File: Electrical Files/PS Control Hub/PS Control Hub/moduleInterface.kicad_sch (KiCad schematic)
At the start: 4 parts, among them K1 Relay_SPST-NO

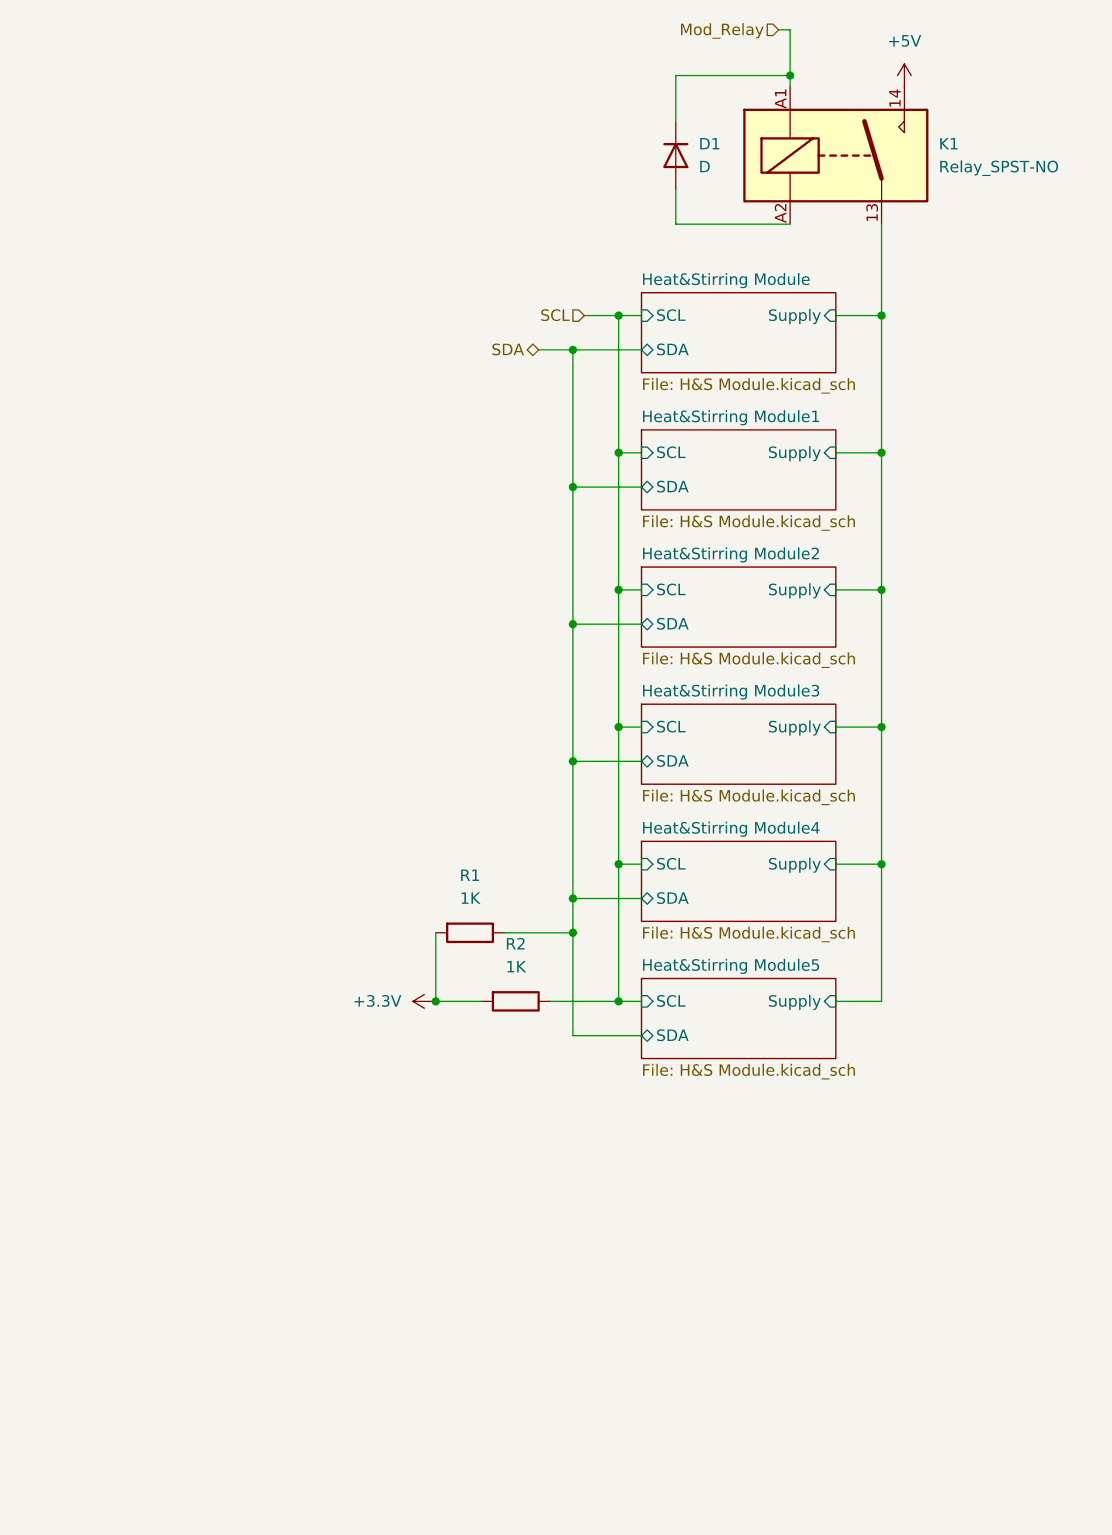
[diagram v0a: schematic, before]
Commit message: Control Hub, Flexible Hotplate, Housing Fan
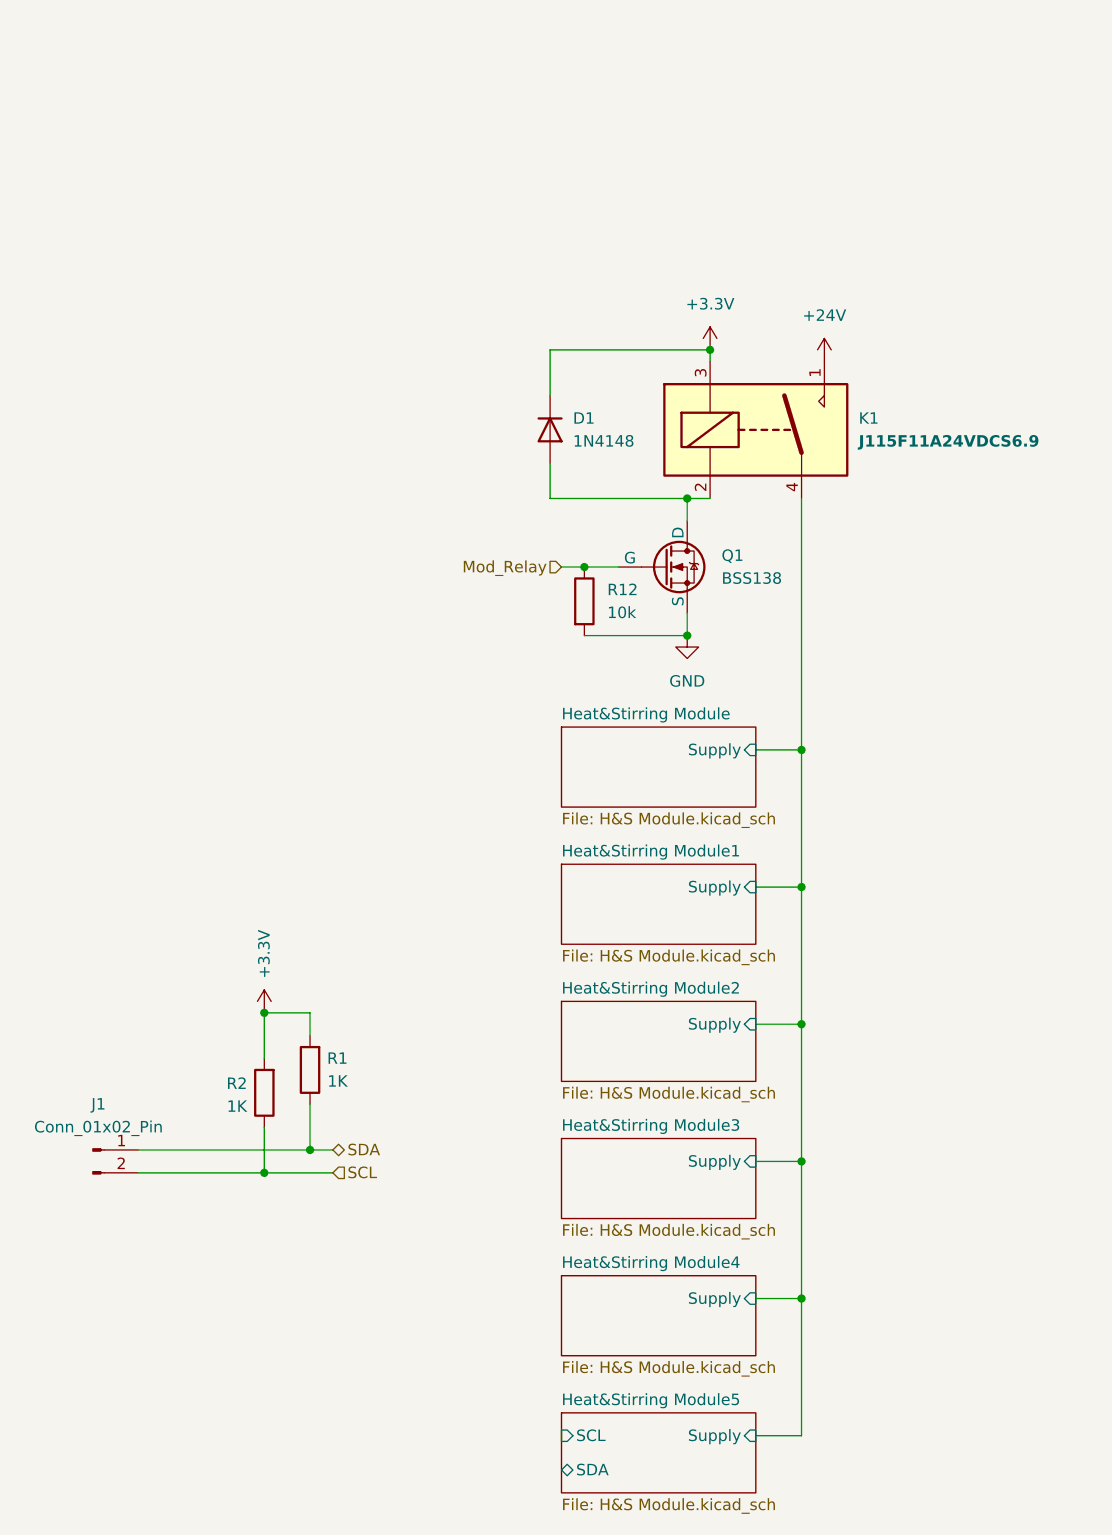
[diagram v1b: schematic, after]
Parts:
- added J1: Conn_01x02_Pin, Connector_Molex:Molex_Mini-Fit_Jr_5566-02A_2x01_P4.20mm_Vertical, symbol Connector:Conn_01x02_Pin
- added Q1: BSS138, Package_TO_SOT_SMD:SOT-23-3, symbol Simulation_SPICE:NMOS
- added R12: 10k, Resistor_SMD:R_0805_2012Metric_Pad1.20x1.40mm_HandSolder, symbol Device:R
- D1: value D -> 1N4148; footprint (none) -> Diode_THT:D_DO-35_SOD27_P7.62mm_Horizontal
- K1: value Relay_SPST-NO -> J115F11A24VDCS6.9; footprint (none) -> Pozzo Lab:J115F1_1A_S_6_CRS
- R1, R2: footprint (none) -> Resistor_SMD:R_0805_2012Metric_Pad1.20x1.40mm_HandSolder
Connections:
- net +3.3V: now also D1.1 (K), K1.3
- net Heat&Stirring Module/Supply: now also K1.4; no longer K1.13
- net Mod_Relay: now also Q1.2 (G), R12.1; no longer D1.1 (K), K1.A1
- net SCL: now also J1.2 (Pin_2)
- net SDA: now also J1.1 (Pin_1)
- net at D1.2 (A): now also K1.2, Q1.1 (D); no longer K1.A2
- removed net +5V: K1.14
- new net +24V: K1.1
- new net GND: Q1.3 (S), R12.2
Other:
- sheet Heat&Stirring Module ports: added none; removed SCL, SDA
- sheet Heat&Stirring Module1 ports: added none; removed SCL, SDA
- sheet Heat&Stirring Module2 ports: added none; removed SCL, SDA
- sheet Heat&Stirring Module3 ports: added none; removed SCL, SDA
- sheet Heat&Stirring Module4 ports: added none; removed SCL, SDA
- moved on the sheet: D1, K1, R1, R2
